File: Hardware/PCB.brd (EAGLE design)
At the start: 170.3 x 111.2 mm, 103 parts, among them IC1 BD5229G-TR, IC4 XC6220A331MR-G, J1 FH34SRJ-24S-0.5SH_99_, J2 SAMACSYS_PARTS_USB4110-GF-A, J3 QWIIC_RIGHT_ANGLE, J4 112A-TAAR-R03_ATTEND, Q1 20V/4.2A/52mΩ/1.4W, Q2 20V/4.2A/52mΩ/1.4W, Q3 SI1308EDL-T1-GE3, U1 W25Q512JVEIQ, U2 ESP32-C6-WROOM-1-N8, U3 DS3231SN#, U4 MAX17048G+T10

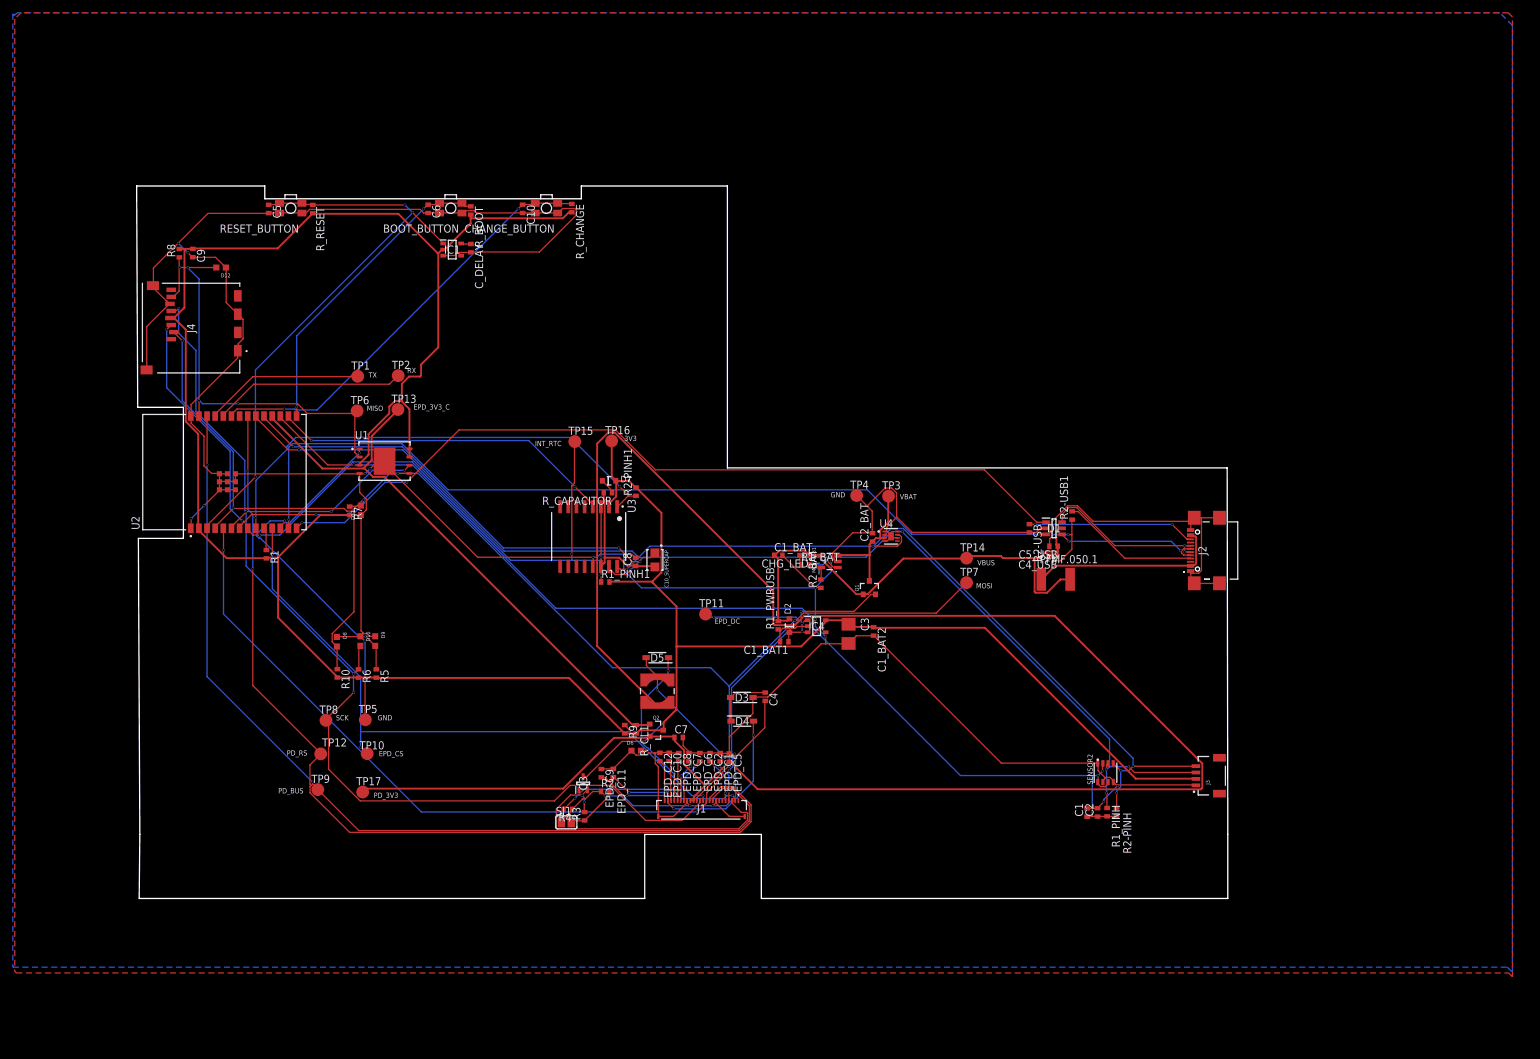
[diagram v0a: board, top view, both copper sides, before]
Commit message: Resolved the raised issues
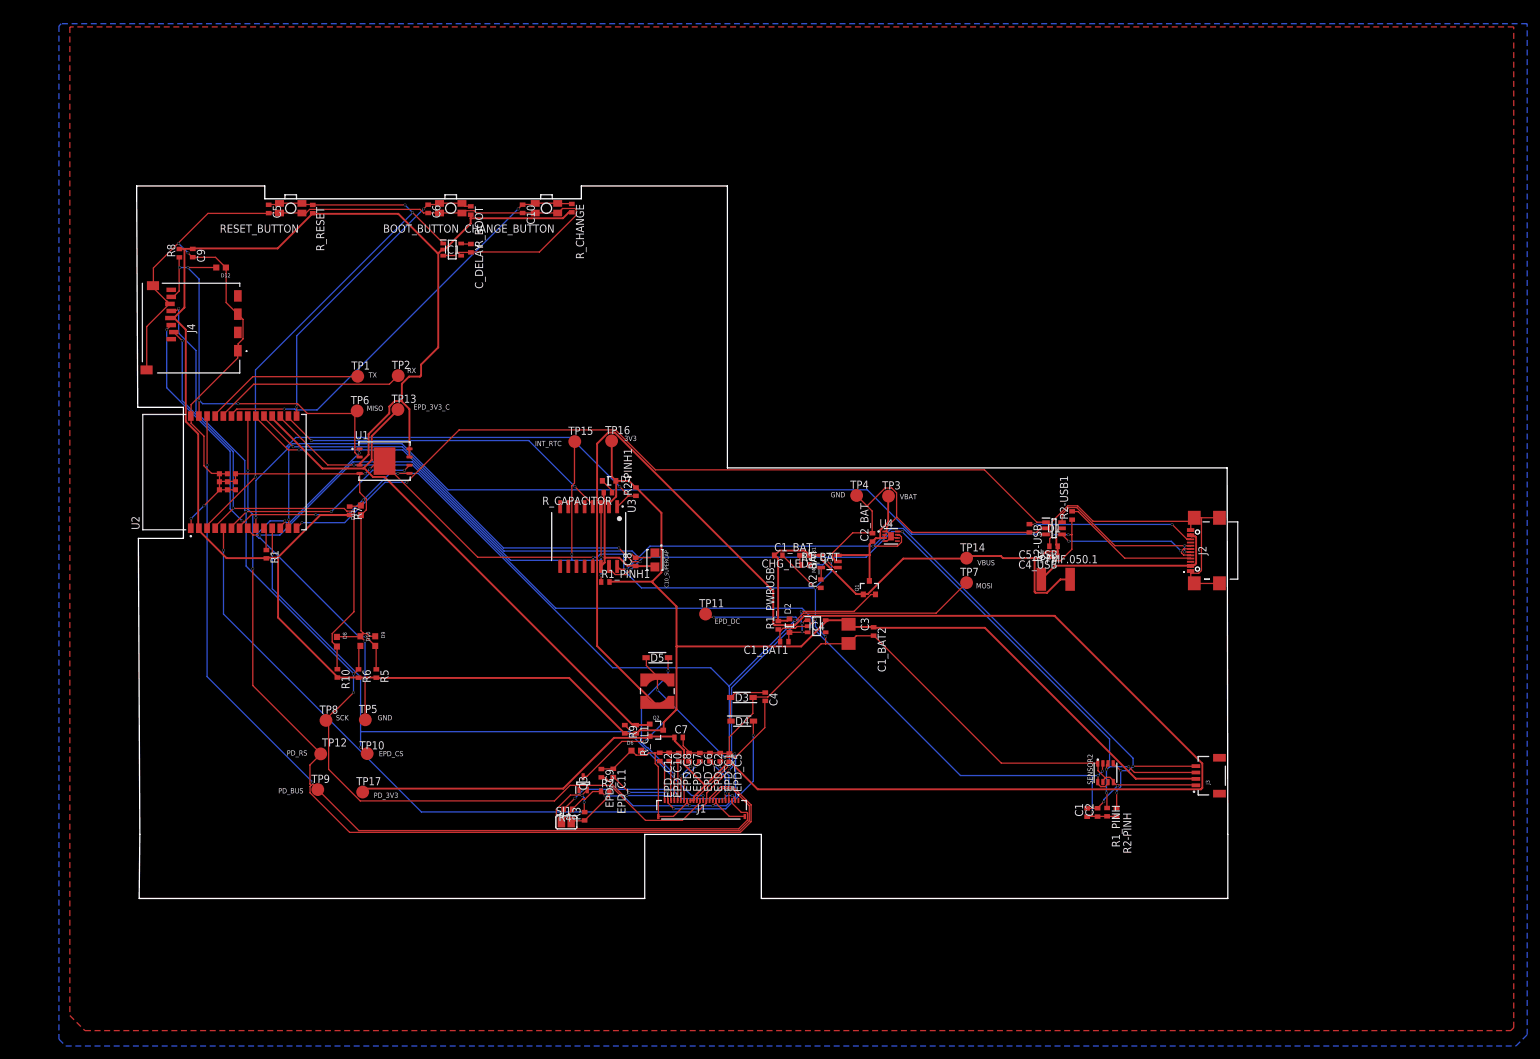
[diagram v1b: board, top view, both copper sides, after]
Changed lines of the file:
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@@
 </via>
 <polygon width="0.1524" layer="1" spacing="1.27" pour="solid" thermals="yes">
-<vertex x="213.71515625" y="-11.6238"/>
-<vertex x="213.7431625" y="-11.6354"/>
-<vertex x="214.3238" y="-12.2160375"/>
-<vertex x="214.3238" y="137.5684375"/>
-<vertex x="213.6684375" y="138.2238"/>
-<vertex x="-18.4684375" y="138.2238"/>
-<vertex x="-19.4238" y="137.2684375"/>
-<vertex x="-19.4238" y="-11.3684375"/>
-<vertex x="-19.1684375" y="-11.6238"/>
+<vertex x="-8.4684375" y="-20.6238"/>
+<vertex x="214.0684375" y="-20.6238"/>
+<vertex x="214.5238" y="-20.1684375"/>
+<vertex x="214.5238" y="136.0238"/>
+<vertex x="-10.8238" y="136.0238"/>
+<vertex x="-10.8238" y="-18.2684375"/>
 </polygon>
 <polygon width="0.1524" layer="16" spacing="1.27" pour="solid" thermals="yes">
-<vertex x="213.51515625" y="-10.7238"/>
-<vertex x="213.5431625" y="-10.7354"/>
-<vertex x="214.3238" y="-11.5160375"/>
-<vertex x="214.3238" y="136.2684375"/>
-<vertex x="212.3684375" y="138.2238"/>
-<vertex x="-19.0684375" y="138.2238"/>
-<vertex x="-19.439321875" y="137.852915625"/>
-<vertex x="-19.442153125" y="137.848134375"/>
-<vertex x="-19.44995" y="137.8422875"/>
-<vertex x="-19.4568375" y="137.8354"/>
-<vertex x="-19.46196875" y="137.833275"/>
-<vertex x="-19.46640625" y="137.829946875"/>
-<vertex x="-19.4758375" y="137.82753125"/>
-<vertex x="-19.48484375" y="137.8238"/>
-<vertex x="-19.49039375" y="137.8238"/>
-<vertex x="-19.495771875" y="137.822421875"/>
-<vertex x="-19.50541875" y="137.8238"/>
-<vertex x="-19.51515625" y="137.8238"/>
-<vertex x="-19.520284375" y="137.825925"/>
-<vertex x="-19.52578125" y="137.826709375"/>
-<vertex x="-19.534165625" y="137.831675"/>
-<vertex x="-19.5431625" y="137.8354"/>
-<vertex x="-19.547084375" y="137.839321875"/>
-<vertex x="-19.551865625" y="137.842153125"/>
-<vertex x="-19.557715625" y="137.849953125"/>
-<vertex x="-19.5646" y="137.8568375"/>
-<vertex x="-19.566721875" y="137.8619625"/>
-<vertex x="-19.7238" y="138.0714"/>
-<vertex x="-19.7238" y="-10.7238"/>
+<vertex x="-11.4684375" y="-23.0238"/>
+<vertex x="214.8684375" y="-23.0238"/>
+<vertex x="216.6238" y="-21.2684375"/>
+<vertex x="216.6238" y="136.5238"/>
+<vertex x="-12.1684375" y="136.5238"/>
+<vertex x="-12.5238" y="136.1684375"/>
+<vertex x="-12.5238" y="-21.9684375"/>
 </polygon>
 </signal>
